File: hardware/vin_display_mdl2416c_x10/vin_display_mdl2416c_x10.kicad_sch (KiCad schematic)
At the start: 51 parts, among them J1 DEBUG, J2 USB_B_Micro, J3 DEBUG_UART, J4 IF_UART, J5 AUX_CONNECTOR, Q1 BSS138, SW1 SW_RESET, SW2 BOOTSEL, SW3 KNOB, U1 W25Q16JVSNIQ, U2 MIC23050-SYML, U3 RP2040, U4 HEF4028BT, X1 12MHz

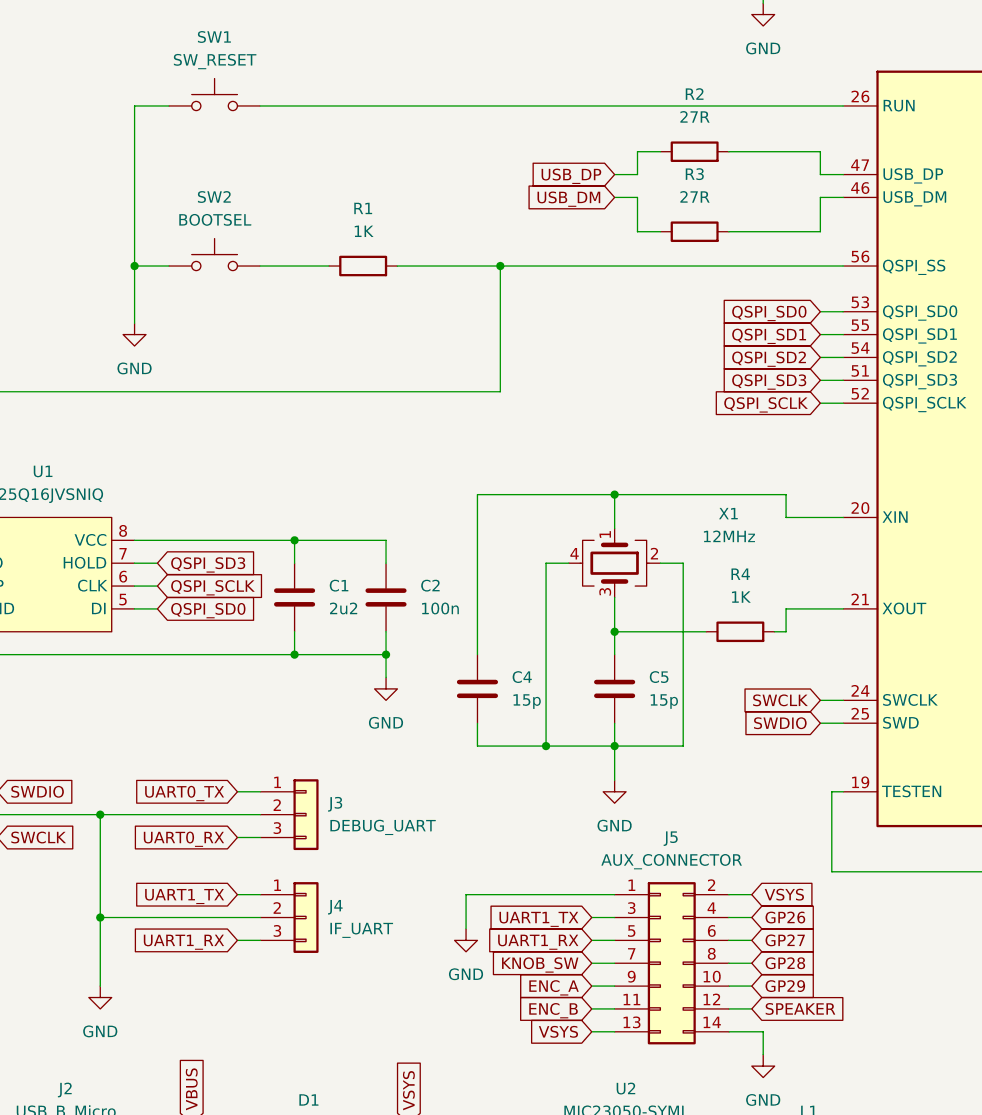
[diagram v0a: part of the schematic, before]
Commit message: work on pcb layout
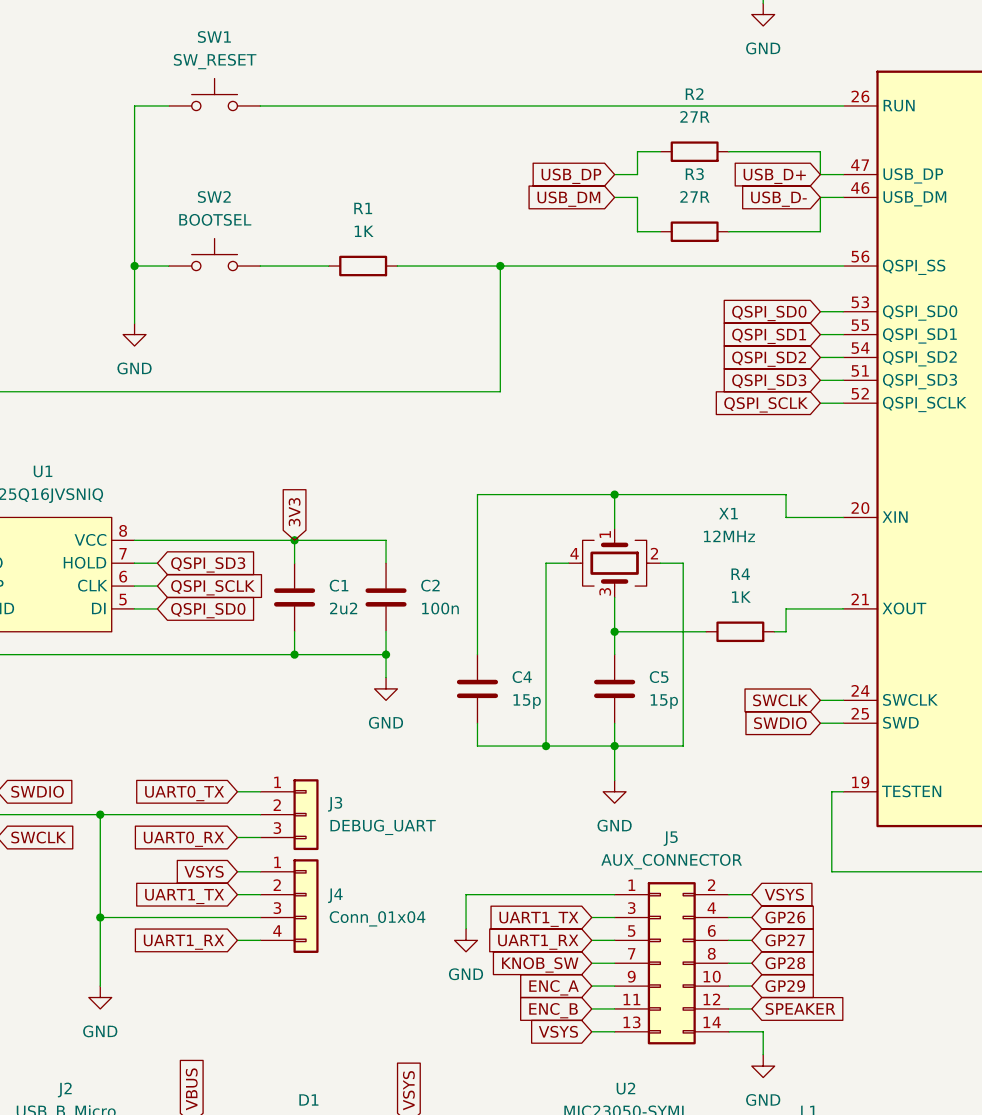
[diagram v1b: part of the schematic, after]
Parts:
- removed J4: IF_UART, Connector_PinHeader_2.54mm:PinHeader_1x03_P2.54mm_Vertical, symbol Connector_Generic:Conn_01x03
- added J4: Conn_01x04, Connector_PinHeader_2.54mm:PinHeader_1x04_P2.54mm_Vertical, symbol Connector_Generic:Conn_01x04
- U2: footprint Package_DFN_QFN:Micrel_MLF-8-1EP_2x2mm_P0.5mm_EP0.6x1.2mm_ThermalVias -> Package_DFN_QFN:Micrel_MLF-8-1EP_2x2mm_P0.5mm_EP0.6x1.2mm
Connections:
- net 3V3: now also C1.1, C2.1, U1.8 (VCC)
- net GND: now also J4.3 (Pin_3)
- net UART1_RX: now also J4.4 (Pin_4)
- net UART1_TX: now also J4.2 (Pin_2)
- net VSYS: now also J4.1 (Pin_1)
- net USB_D-: now reaches R3.2, U3.46 (USB_DM)
- net USB_D+: now reaches R2.2, U3.47 (USB_DP)
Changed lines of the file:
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@@
+    (stroke (width 0) (type default) (color 0 0 0 0))
+  )
+  (wire (pts (xy 60.96 134.62) (xy 63.5 134.62))
     (stroke (width 0) (type default) (color 0 0 0 0))
   )
@@
     )
   )
+  (global_label "3V3" (shape input) (at 67.31 97.79 90) (fields_autoplaced)
+    (effects (font (size 1.27 1.27)) (justify left))
+    (property "Intersheet References" "${INTERSHEET_REFS}" (id 0) (at 67.2306 91.8693 90)
+      (effects (font (size 1.27 1.27)) (justify left) hide)
+    )
+  )
   (global_label "VBUS" (shape input) (at 55.88 162.56 90) (fields_autoplaced)
     (effects (font (size 1.27 1.27)) (justify left))
@@
     (property "Intersheet References" "${INTERSHEET_REFS}" (id 0) (at 193.0341 59.6106 0)
       (effects (font (size 1.27 1.27)) (justify left) hide)
+    )
+  )
+  (global_label "USB_D-" (shape input) (at 125.73 59.69 180) (fields_autoplaced)
+    (effects (font (size 1.27 1.27)) (justify right))
+    (property "Intersheet References" "${INTERSHEET_REFS}" (id 0) (at 115.6969 59.6106 0)
+      (effects (font (size 1.27 1.27)) (justify right) hide)
     )
   )
@@
     (effects (font (size 1.27 1.27)) (justify right))
     (property "Intersheet References" "${INTERSHEET_REFS}" (id 0) (at 114.2455 72.4694 0)
+      (effects (font (size 1.27 1.27)) (justify right) hide)
+    )
+  )
+  (global_label "USB_D+" (shape input) (at 125.73 57.15 180) (fields_autoplaced)
+    (effects (font (size 1.27 1.27)) (justify right))
+    (property "Intersheet References" "${INTERSHEET_REFS}" (id 0) (at 115.6969 57.0706 0)
+      (effects (font (size 1.27 1.27)) (justify right) hide)
+    )
+  )
+  (global_label "VSYS" (shape input) (at 60.96 134.62 180) (fields_autoplaced)
+    (effects (font (size 1.27 1.27)) (justify right))
+    (property "Intersheet References" "${INTERSHEET_REFS}" (id 0) (at 53.9507 134.5406 0)
       (effects (font (size 1.27 1.27)) (justify right) hide)
     )
@@
     )
     (property "Datasheet" "~" (id 3) (at 26.67 128.27 0)
-      (effects (font (size 1.27 1.27)) hide)
-    )
-    (pin "1")
-    (pin "2")
-    (pin "3")
-  )
-  (symbol (lib_id "Connector_Generic:Conn_01x03") (at 68.58 139.7 0) (unit 1)
-    (in_bom yes) (on_board yes) (fields_autoplaced)
-    (property "Reference" "J4" (id 0) (at 71.12 138.4299 0)
-      (effects (font (size 1.27 1.27)) (justify left))
-    )
-    (property "Value" "IF_UART" (id 1) (at 71.12 140.9699 0)
-      (effects (font (size 1.27 1.27)) (justify left))
-    )
-    (property "Footprint" "Connector_PinHeader_2.54mm:PinHeader_1x03_P2.54mm_Vertical" (id 2) (at 68.58 139.7 0)
-      (effects (font (size 1.27 1.27)) hide)
-    )
-    (property "Datasheet" "~" (id 3) (at 68.58 139.7 0)
       (effects (font (size 1.27 1.27)) hide)
     )
@@
     (pin "2")
   )
+  (symbol (lib_id "Connector_Generic:Conn_01x04") (at 68.58 137.16 0) (unit 1)
+    (in_bom yes) (on_board yes) (fields_autoplaced)
+    (property "Reference" "J4" (id 0) (at 71.12 137.1599 0)
+      (effects (font (size 1.27 1.27)) (justify left))
+    )
+    (property "Value" "Conn_01x04" (id 1) (at 71.12 139.6999 0)
+      (effects (font (size 1.27 1.27)) (justify left))
+    )
+    (property "Footprint" "Connector_PinHeader_2.54mm:PinHeader_1x04_P2.54mm_Vertical" (id 2) (at 68.58 137.16 0)
+      (effects (font (size 1.27 1.27)) hide)
+    )
+    (property "Datasheet" "~" (id 3) (at 68.58 137.16 0)
+      (effects (font (size 1.27 1.27)) hide)
+    )
+    (pin "1")
+    (pin "2")
+    (pin "3")
+    (pin "4")
+  )
   (symbol (lib_id "Device:R") (at 111.76 54.61 90) (unit 1)
     (in_bom yes) (on_board yes) (fields_autoplaced)
@@
     (property "Reference" "U2" (id 0) (at 104.14 158.75 0))
     (property "Value" "MIC23050-SYML" (id 1) (at 104.14 161.29 0))
-    (property "Footprint" "Package_DFN_QFN:Micrel_MLF-8-1EP_2x2mm_P0.5mm_EP0.6x1.2mm_ThermalVias" (id 2) (at 109.22 170.18 0)
+    (property "Footprint" "Package_DFN_QFN:Micrel_MLF-8-1EP_2x2mm_P0.5mm_EP0.6x1.2mm" (id 2) (at 109.22 170.18 0)
       (effects (font (size 1.27 1.27)) (justify left) hide)
     )
@@
       (reference "J3") (unit 1) (value "DEBUG_UART") (footprint "Connector_PinHeader_2.54mm:PinHeader_1x03_P2.54mm_Vertical")
     )
-    (path "/52948f66-709e-42ba-95a6-a598f591e63a"
-      (reference "J4") (unit 1) (value "IF_UART") (footprint "Connector_PinHeader_2.54mm:PinHeader_1x03_P2.54mm_Vertical")
+    (path "/83b99386-65f3-4d5f-ace0-dfc7848335c3"
+      (reference "J4") (unit 1) (value "Conn_01x04") (footprint "Connector_PinHeader_2.54mm:PinHeader_1x04_P2.54mm_Vertical")
     )
     (path "/24dea3f5-faa1-4f14-a163-ea0dcc26d440"
@@
     )
     (path "/fc845537-7277-43cf-9d22-ef1876c41284"
-      (reference "U2") (unit 1) (value "MIC23050-SYML") (footprint "Package_DFN_QFN:Micrel_MLF-8-1EP_2x2mm_P0.5mm_EP0.6x1.2mm_ThermalVias")
+      (reference "U2") (unit 1) (value "MIC23050-SYML") (footprint "Package_DFN_QFN:Micrel_MLF-8-1EP_2x2mm_P0.5mm_EP0.6x1.2mm")
     )
     (path "/73b74445-0b4c-42ed-8ac5-ea72e30c4bc1"
